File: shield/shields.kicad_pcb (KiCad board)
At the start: 2 copper layers, 40.4 x 95.7 mm, 1 part

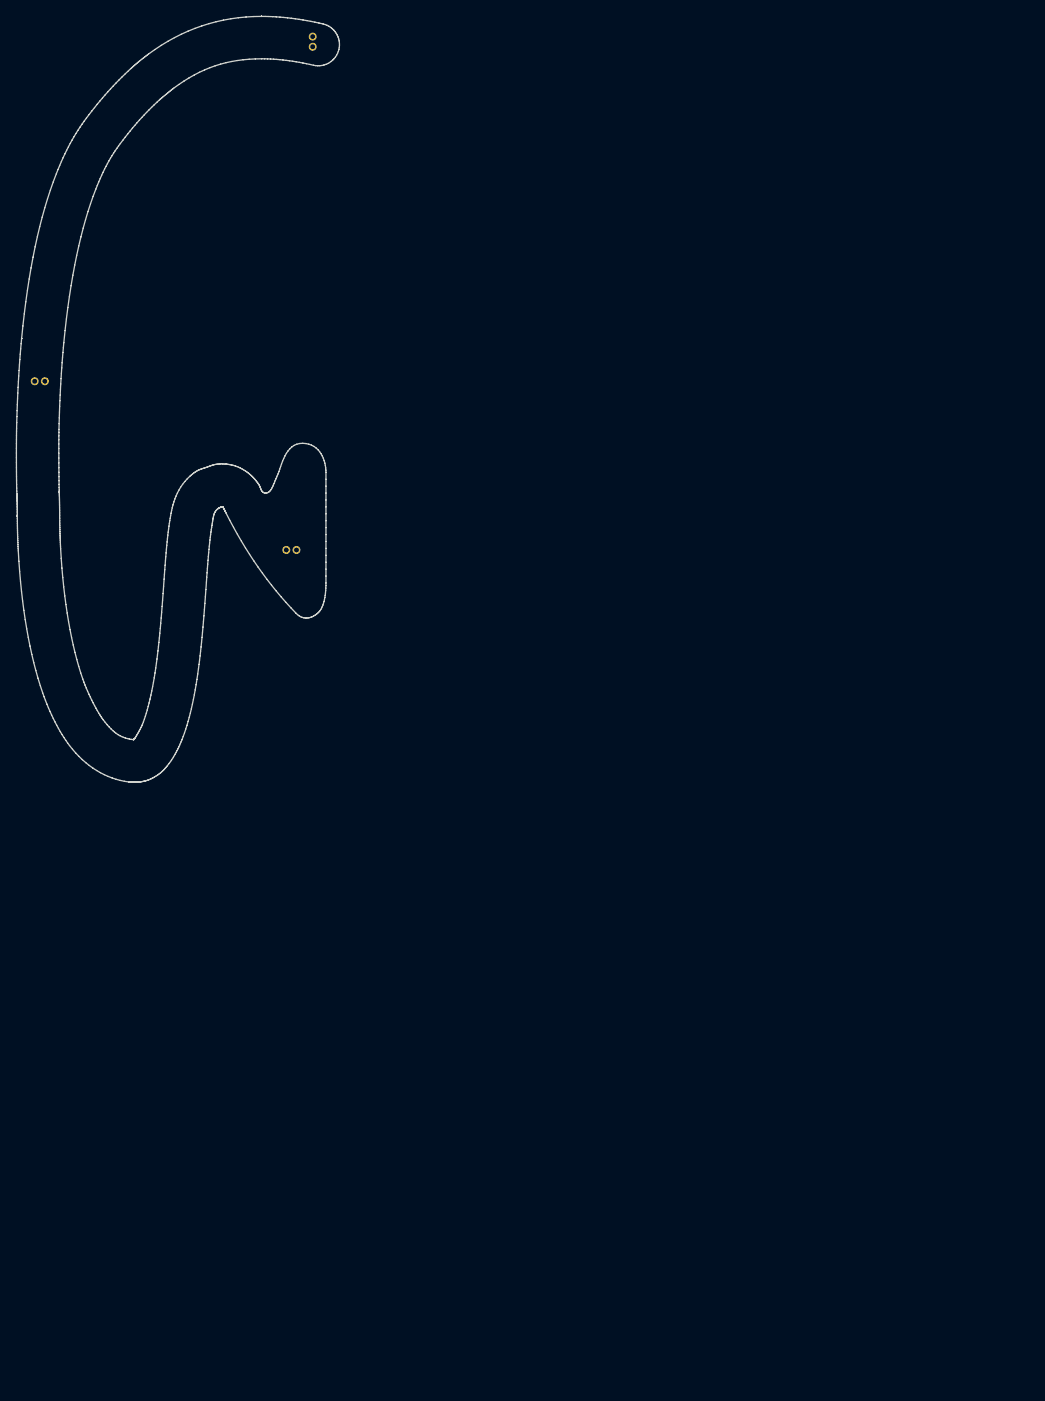
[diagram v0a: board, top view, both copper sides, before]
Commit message: Update as ordered.
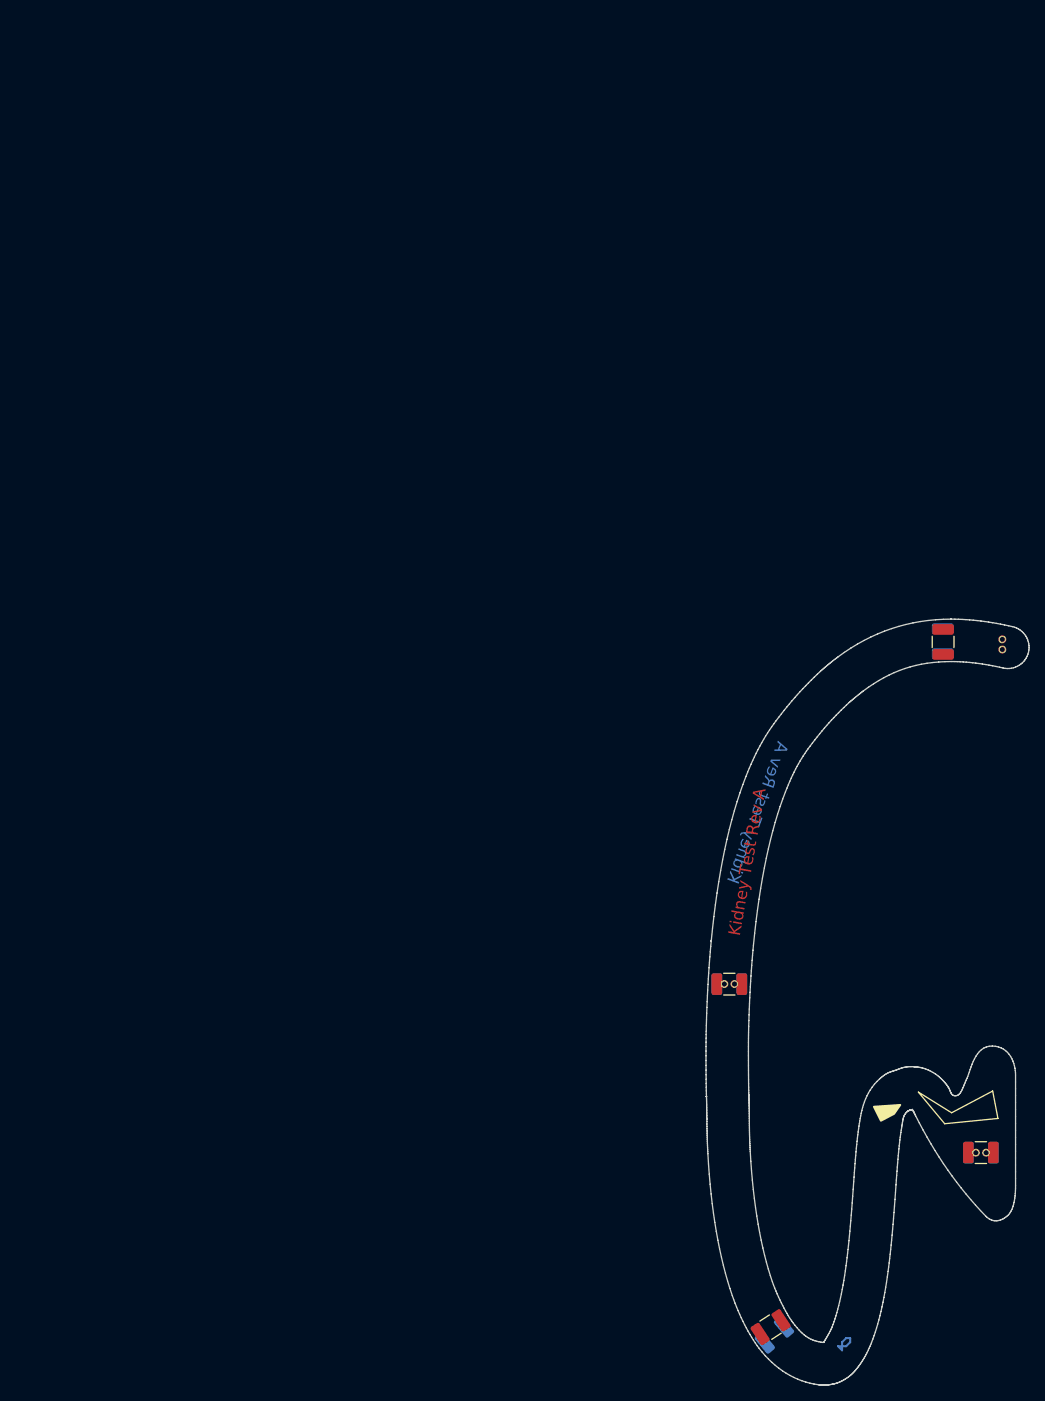
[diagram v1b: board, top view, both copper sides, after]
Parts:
- added REF**: C_1210_3225Metric_Pad1.33x2.70mm_HandSolder, Swadge_Parts:C_1210_3225Metric_Pad1.33x2.70mm_HandSolder, F.Cu at (28.7, 116.0)
- added REF**: C_1210_3225Metric_Pad1.33x2.70mm_HandSolder, Swadge_Parts:C_1210_3225Metric_Pad1.33x2.70mm_HandSolder, F.Cu at (23.5, 73.1)
- added REF**: C_1210_3225Metric_Pad1.33x2.70mm_HandSolder, Swadge_Parts:C_1210_3225Metric_Pad1.33x2.70mm_HandSolder, F.Cu at (50.2, 30.3)
- added REF**: C_1210_3225Metric_Pad1.33x2.70mm_HandSolder, Swadge_Parts:C_1210_3225Metric_Pad1.33x2.70mm_HandSolder, F.Cu at (54.9, 94.2)
- added REF**: C_1210_3225Metric_Pad1.33x2.70mm_HandSolder, Swadge_Parts:C_1210_3225Metric_Pad1.33x2.70mm_HandSolder, B.Cu at (55.0, 94.2)
- added REF**: C_1210_3225Metric_Pad1.33x2.70mm_HandSolder, Swadge_Parts:C_1210_3225Metric_Pad1.33x2.70mm_HandSolder, B.Cu at (29.1, 116.9)
- added REF**: C_1210_3225Metric_Pad1.33x2.70mm_HandSolder, Swadge_Parts:C_1210_3225Metric_Pad1.33x2.70mm_HandSolder, B.Cu at (50.2, 30.2)
- added REF**: C_1210_3225Metric_Pad1.33x2.70mm_HandSolder, Swadge_Parts:C_1210_3225Metric_Pad1.33x2.70mm_HandSolder, B.Cu at (23.5, 73.1)
- moved Ref** 114.5 mm to (86.2, 75.3)
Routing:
- net (no net): track 0.00 -> 5.20 mm
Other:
- rule pad_to_mask_clearance: 0.2 -> 0
- board text added: "Fab notes: 0.6mm Thick FR4"
- board text added: "Kidney Test Rev A"
